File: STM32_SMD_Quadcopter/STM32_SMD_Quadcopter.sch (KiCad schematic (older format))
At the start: 64 parts, among them J1 PWR, J2 USB_B_Micro, J3 Micro_SD_Card_Det, J4 DEBUG, J5 DSMX, M1 Brushed_DC, M2 Brushed_DC, M3 Brushed_DC, M4 Brushed_DC, Q1 IRLML6244TR, Q2 IRLML6244TR, Q3 IRLML6244TR, Q4 IRLML6244TR, SW1 SW_Push, U1 AMS1117-3.3, U3 FT230XQ, U4 STM32F446RETx, U5 MPU-6050, Y1 16MHz X322516MLB4SI

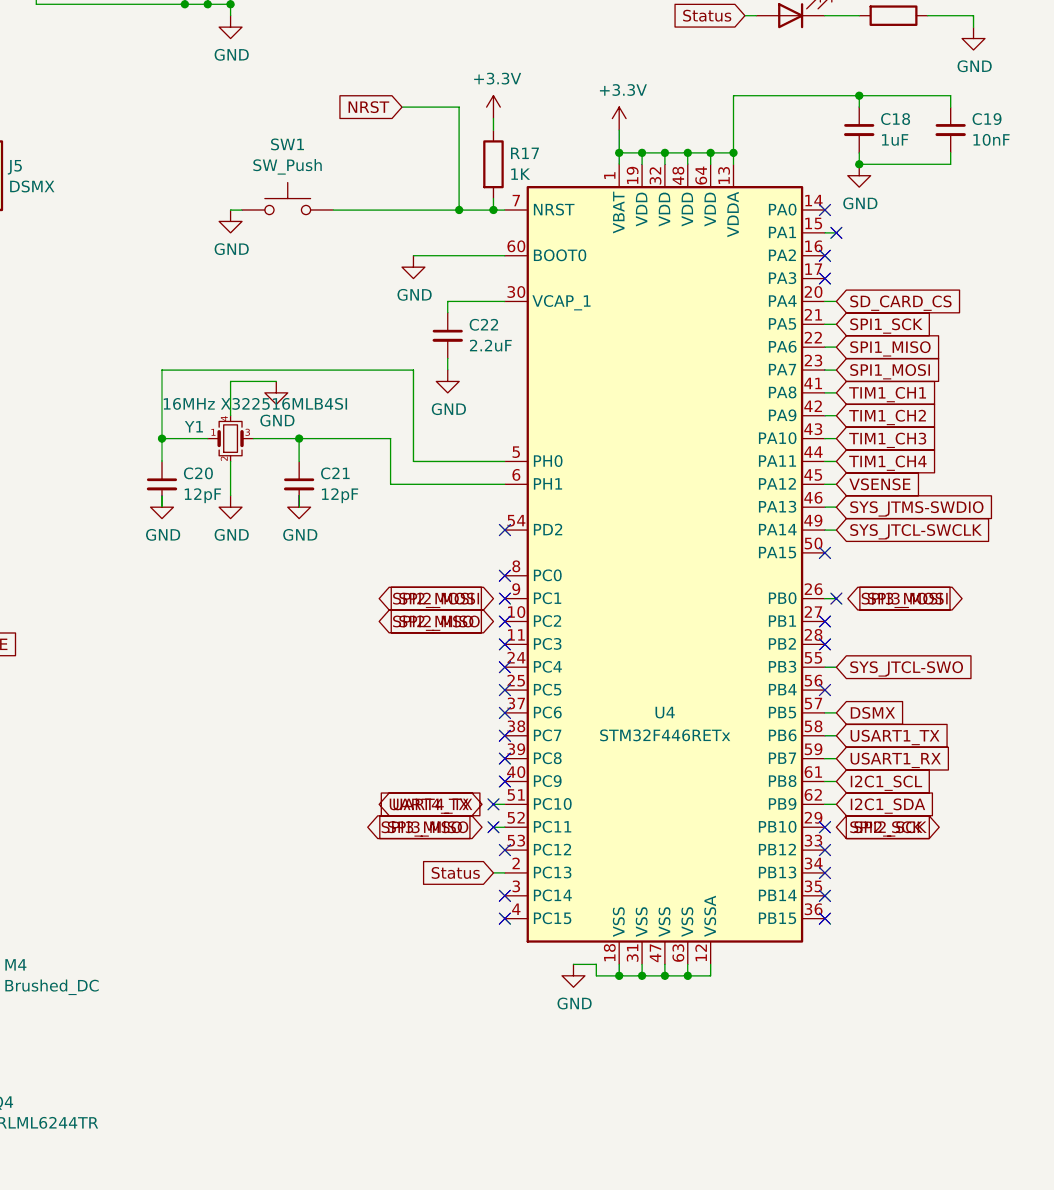
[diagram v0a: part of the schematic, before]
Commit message: Purchase version
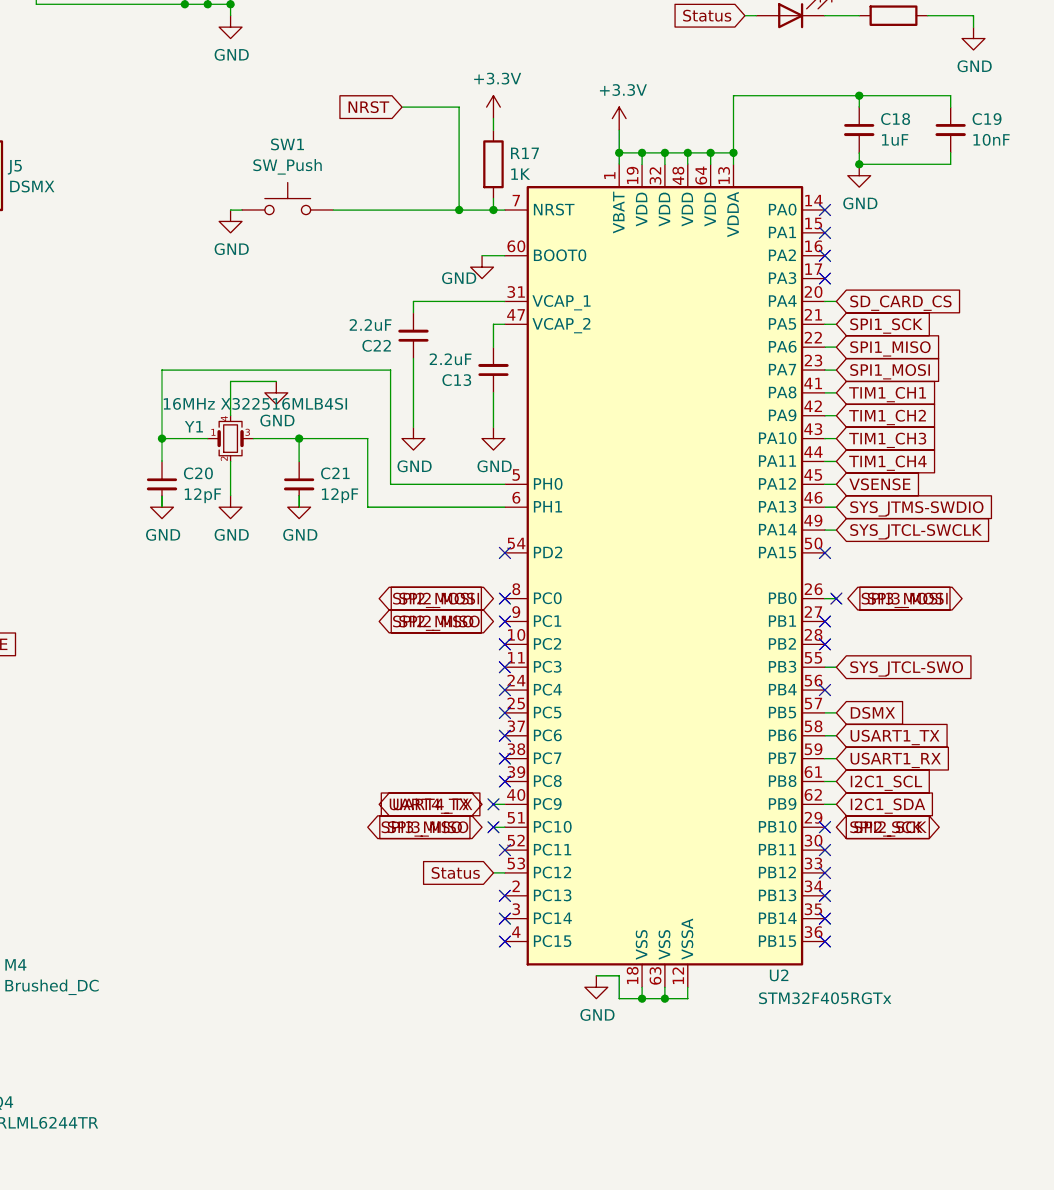
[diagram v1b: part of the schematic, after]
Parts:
- removed U4: STM32F446RETx, Package_QFP:LQFP-64_10x10mm_P0.5mm, symbol MCU_ST_STM32F4:STM32F446RETx
- added C13: 2.2uF, Capacitor_SMD:C_0603_1608Metric, symbol Device:C_Small
- added U2: STM32F405RGTx, Package_QFP:LQFP-64_10x10mm_P0.5mm, symbol MCU_ST_STM32F4:STM32F405RGTx
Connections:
- net +3V3: now also U2.1 (VBAT), U2.13 (VDDA), U2.19 (VDD), U2.32 (VDD), U2.48 (VDD), U2.64 (VDD)
- net DSMX: now also U2.57 (PB5)
- net GND: now also C22.1, C13.1, U2.12 (VSSA), U2.18 (VSS), U2.60 (BOOT0), U2.63 (VSS); no longer C22.2
- net I2C1_SCL: now also U2.61 (PB8)
- net I2C1_SDA: now also U2.62 (PB9)
- net MOTOR_A: now also U2.42 (PA9)
- net MOTOR_B: now also U2.41 (PA8)
- net MOTOR_C: now also U2.44 (PA11)
- net MOTOR_D: now also U2.43 (PA10)
- net NRST: now also U2.7 (NRST)
- net SD_CARD_CS: now also U2.20 (PA4)
- net SPI1_MISO: now also U2.22 (PA6)
- net SPI1_MOSI: now also U2.23 (PA7)
- net SPI1_SCK: now also U2.21 (PA5)
- net SYS_JTCL-SWCLK: now also U2.49 (PA14)
- net SYS_JTCL-SWO: now also U2.55 (PB3)
- net SYS_JTMS-SWDIO: now also U2.46 (PA13)
- net Status: now also U2.53 (PC12)
- net USART1_RX: now also U2.59 (PB7)
- net USART1_TX: now also U2.58 (PB6)
- net VSENSE: now also U2.45 (PA12)
- net at C20.1, Y1.1: now also U2.5 (PH0)
- net at C21.1, Y1.3: now also U2.6 (PH1)
- new net: C22.2, U2.31 (VCAP_1)
- new net: C13.2, U2.47 (VCAP_2)
- no-connect marks 44 -> 45
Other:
- moved on the sheet: C22
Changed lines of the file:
@@
-$EndComp
-$Comp
-L MCU_ST_STM32F4:STM32F446RETx U4
-U 1 1 5D1D966A
-P 8900 4700
-F 0 "U4" H 8900 4000 50  0000 C CNN
-F 1 "STM32F446RETx" H 8900 3900 50  0000 C CNN
-F 2 "Package_QFP:LQFP-64_10x10mm_P0.5mm" H 8300 3000 50  0001 R CNN
-F 3 "http://www.st.com/st-web-ui/static/active/en/resource/technical/document/datasheet/DM00141306.pdf" H 8900 4700 50  0001 C CNN
-F 4 "C69336" H 8900 4700 50  0001 C CNN "LCSC Part #"
-F 5 "C69336" H 8900 4700 50  0001 C CNN "LCSC"
-	1    8900 4700
-	1    0    0    -1
 $EndComp
 $Comp
@@
 Wire Wire Line
 	6700 4450 6700 4500
-Wire Wire Line
-	7800 3400 8200 3400
 $Comp
 L Device:C_Small C22
 U 1 1 5D24D0EE
-P 7950 3750
-F 0 "C22" H 8042 3796 50  0000 L CNN
-F 1 "2.2uF" H 8042 3705 50  0000 L CNN
-F 2 "Capacitor_SMD:C_0603_1608Metric" H 7950 3750 50  0001 C CNN
-F 3 "~" H 7950 3750 50  0001 C CNN
-F 4 "C23630" H 7950 3750 50  0001 C CNN "LCSC Part #"
-F 5 "C23630" H 7950 3750 50  0001 C CNN "LCSC"
-	1    7950 3750
-	1    0    0    -1
+P 7800 3750
+F 0 "C22" H 7892 3796 50  0000 L CNN
+F 1 "2.2uF" H 7892 3705 50  0000 L CNN
+F 2 "Capacitor_SMD:C_0603_1608Metric" H 7800 3750 50  0001 C CNN
+F 3 "~" H 7800 3750 50  0001 C CNN
+F 4 "C23630" H 7800 3750 50  0001 C CNN "LCSC Part #"
+F 5 "C23630" H 7800 3750 50  0001 C CNN "LCSC"
+	1    7800 3750
+	-1   0    0    1
 $EndComp
 $Comp
 L power:GND #PWR040
 U 1 1 5D24D318
-P 7950 3900
-F 0 "#PWR040" H 7950 3650 50  0001 C CNN
-F 1 "GND" H 7955 3727 50  0000 C CNN
-F 2 "" H 7950 3900 50  0001 C CNN
-F 3 "" H 7950 3900 50  0001 C CNN
-	1    7950 3900
-	1    0    0    -1
-$EndComp
-Wire Wire Line
-	7950 3900 7950 3850
+P 7800 4150
+F 0 "#PWR040" H 7800 3900 50  0001 C CNN
+F 1 "GND" H 7805 3977 50  0000 C CNN
+F 2 "" H 7800 4150 50  0001 C CNN
+F 3 "" H 7800 4150 50  0001 C CNN
+	1    7800 4150
+	1    0    0    -1
+$EndComp
+Wire Wire Line
+	7800 4150 7800 3850
 Wire Wire Line
 	8700 3000 8700 2950
@@
 Connection ~ 9100 2950
 Connection ~ 9200 2950
-Wire Wire Line
-	8700 6500 8700 6550
-Wire Wire Line
-	8700 6550 8800 6550
-Wire Wire Line
-	8800 6550 8800 6500
-Wire Wire Line
-	8800 6550 8900 6550
-Wire Wire Line
-	8900 6550 8900 6500
-Connection ~ 8800 6550
-Wire Wire Line
-	8900 6550 9000 6550
-Wire Wire Line
-	9000 6550 9000 6500
-Connection ~ 8900 6550
-Wire Wire Line
-	9100 6550 9100 6500
 $Comp
 L power:+3.3V #PWR045
@@
 	8700 2850 8700 2950
 Connection ~ 8700 2950
-Wire Wire Line
-	9100 6550 9000 6550
-Connection ~ 9000 6550
 $Comp
 L power:GND #PWR044
 U 1 1 5D299679
-P 8500 6500
-F 0 "#PWR044" H 8500 6250 50  0001 C CNN
-F 1 "GND" H 8505 6327 50  0000 C CNN
-F 2 "" H 8500 6500 50  0001 C CNN
-F 3 "" H 8500 6500 50  0001 C CNN
-	1    8500 6500
-	1    0    0    -1
-$EndComp
-Wire Wire Line
-	8500 6500 8600 6500
-Wire Wire Line
-	8600 6500 8600 6550
-Wire Wire Line
-	8600 6550 8700 6550
-Connection ~ 8700 6550
+P 8600 6550
+F 0 "#PWR044" H 8600 6300 50  0001 C CNN
+F 1 "GND" H 8605 6377 50  0000 C CNN
+F 2 "" H 8600 6550 50  0001 C CNN
+F 3 "" H 8600 6550 50  0001 C CNN
+	1    8600 6550
+	1    0    0    -1
+$EndComp
 $Comp
 L Device:C_Small C18
@@
 	9600 4500 9650 4500
 Wire Wire Line
-	9650 3300 9600 3300
-Wire Wire Line
 	9600 3700 9650 3700
 Wire Wire Line
@@
 NoConn ~ 8200 5300
 NoConn ~ 8200 5200
-NoConn ~ 8200 4600
-Wire Wire Line
-	7950 3600 7950 3650
-Wire Wire Line
-	7950 3600 8200 3600
+Wire Wire Line
+	7800 3600 7800 3650
 Wire Wire Line
 	5350 1200 5350 1000
@@
 NoConn ~ 8150 5800
 NoConn ~ 8150 5900
-NoConn ~ 9650 3300
+NoConn ~ 9600 3300
 NoConn ~ 9650 4900
 Text GLabel 1350 2950 0    50   Input ~ 0
@@
 NoConn ~ 9500 1150
 $Comp
-L power:GND #PWR039
-U 1 1 5D233320
-P 7800 3400
-F 0 "#PWR039" H 7800 3150 50  0001 C CNN
-F 1 "GND" H 7805 3227 50  0000 C CNN
-F 2 "" H 7800 3400 50  0001 C CNN
-F 3 "" H 7800 3400 50  0001 C CNN
-	1    7800 3400
-	1    0    0    -1
-$EndComp
-$Comp
 L Device:Crystal_GND24_Small Y1
 U 1 1 5FE60176
@@
 	7200 3950 7000 3950
 Wire Wire Line
-	7800 4300 7800 3900
-Wire Wire Line
-	7800 3900 6700 3900
+	7700 3900 6700 3900
 Wire Wire Line
 	6700 3900 6700 4200
 Wire Wire Line
-	7800 4300 8200 4300
+	7700 4400 8200 4400
 Connection ~ 6700 4200
 Wire Wire Line
-	7300 4200 7700 4200
-Wire Wire Line
-	7700 4200 7700 4400
-Wire Wire Line
-	7700 4400 8200 4400
+	7300 4200 7600 4200
 Connection ~ 7300 4200
 $Comp
@@
 NoConn ~ 8200 4900
 NoConn ~ 8200 5000
-NoConn ~ 8200 4800
 NoConn ~ 9600 5900
 Text GLabel 9550 1050 2    50   Input ~ 0
@@
 	1    0    0    -1
 $EndComp
+$Comp
+L MCU_ST_STM32F4:STM32F405RGTx U2
+U 1 1 60A5CED1
+P 8900 4800
+F 0 "U2" H 9400 3050 50  0000 C CNN
+F 1 "STM32F405RGTx" H 9600 2950 50  0000 C CNN
+F 2 "Package_QFP:LQFP-64_10x10mm_P0.5mm" H 8300 3100 50  0001 R CNN
+F 3 "http://www.st.com/st-web-ui/static/active/en/resource/technical/document/datasheet/DM00037051.pdf" H 8900 4800 50  0001 C CNN
+	1    8900 4800
+	1    0    0    -1
+$EndComp
+Wire Wire Line
+	8600 6550 8700 6550
+Wire Wire Line
+	8700 6550 8700 6650
+Wire Wire Line
+	8700 6650 8800 6650
+Wire Wire Line
+	9000 6650 9000 6600
+Wire Wire Line
+	8900 6600 8900 6650
+Connection ~ 8900 6650
+Wire Wire Line
+	8900 6650 9000 6650
+Wire Wire Line
+	8800 6600 8800 6650
+Connection ~ 8800 6650
+Wire Wire Line
+	8800 6650 8900 6650
+Wire Wire Line
+	7700 3900 7700 4400
+Wire Wire Line
+	8200 4500 7600 4500
+Wire Wire Line
+	7600 4200 7600 4500
+NoConn ~ 8200 4700
+NoConn ~ 9600 6400
+NoConn ~ 8200 6400
+Wire Wire Line
+	7800 3600 8200 3600
+$Comp
+L power:GND #PWR043
+U 1 1 60BD00CD
+P 8150 4150
+F 0 "#PWR043" H 8150 3900 50  0001 C CNN
+F 1 "GND" H 8155 3977 50  0000 C CNN
+F 2 "" H 8150 4150 50  0001 C CNN
+F 3 "" H 8150 4150 50  0001 C CNN
+	1    8150 4150
+	1    0    0    -1
+$EndComp
+$Comp
+L Device:C_Small C13
+U 1 1 60BD1A94
+P 8150 3900
+F 0 "C13" H 8242 3946 50  0000 L CNN
+F 1 "2.2uF" H 8242 3855 50  0000 L CNN
+F 2 "Capacitor_SMD:C_0603_1608Metric" H 8150 3900 50  0001 C CNN
+F 3 "~" H 8150 3900 50  0001 C CNN
+F 4 "C23630" H 8150 3900 50  0001 C CNN "LCSC Part #"
+F 5 "C23630" H 8150 3900 50  0001 C CNN "LCSC"
+	1    8150 3900
+	-1   0    0    1
+$EndComp
+Wire Wire Line
+	8150 3800 8150 3700
+Wire Wire Line
+	8150 3700 8200 3700
+Wire Wire Line
+	8150 4000 8150 4150
+Wire Wire Line
+	8100 3400 8200 3400
+$Comp
+L power:GND #PWR039
+U 1 1 5D233320
+P 8100 3400
+F 0 "#PWR039" H 8100 3150 50  0001 C CNN
+F 1 "GND" H 8000 3300 50  0000 C CNN
+F 2 "" H 8100 3400 50  0001 C CNN
+F 3 "" H 8100 3400 50  0001 C CNN
+	1    8100 3400
+	1    0    0    -1
+$EndComp
